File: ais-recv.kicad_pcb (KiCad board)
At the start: 4 copper layers, 40 x 20 mm, 44 parts, among them J1 Conn_02x05_Odd_Even, J2 CONSMA 003.062, J3 105017-0001, SW1 SW_Push, U1 NCP115ASN330T1G, U2 Si4362-C, U3 STM32L432KCUx, U4 USBLC6-2SC6, U5 Si4362-C, Y1 30 MHz

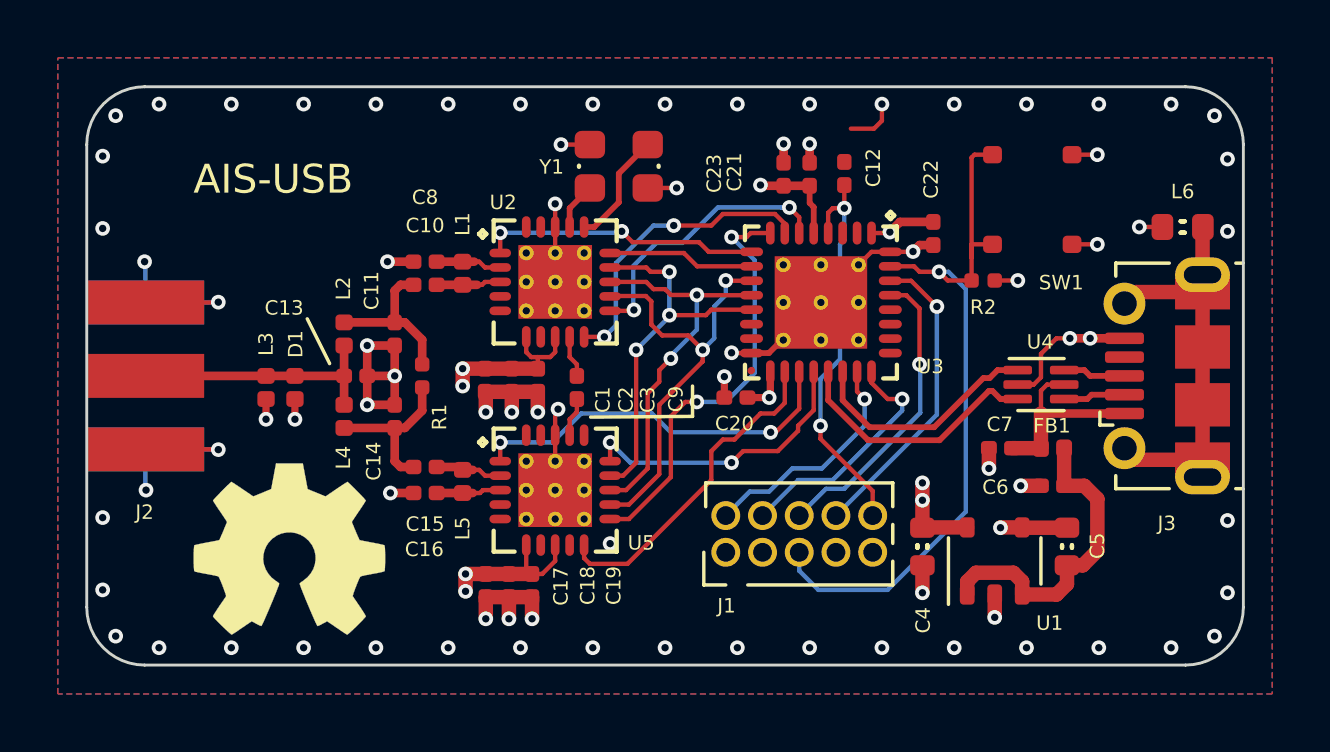
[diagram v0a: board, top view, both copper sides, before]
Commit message: Changes for version 1.0
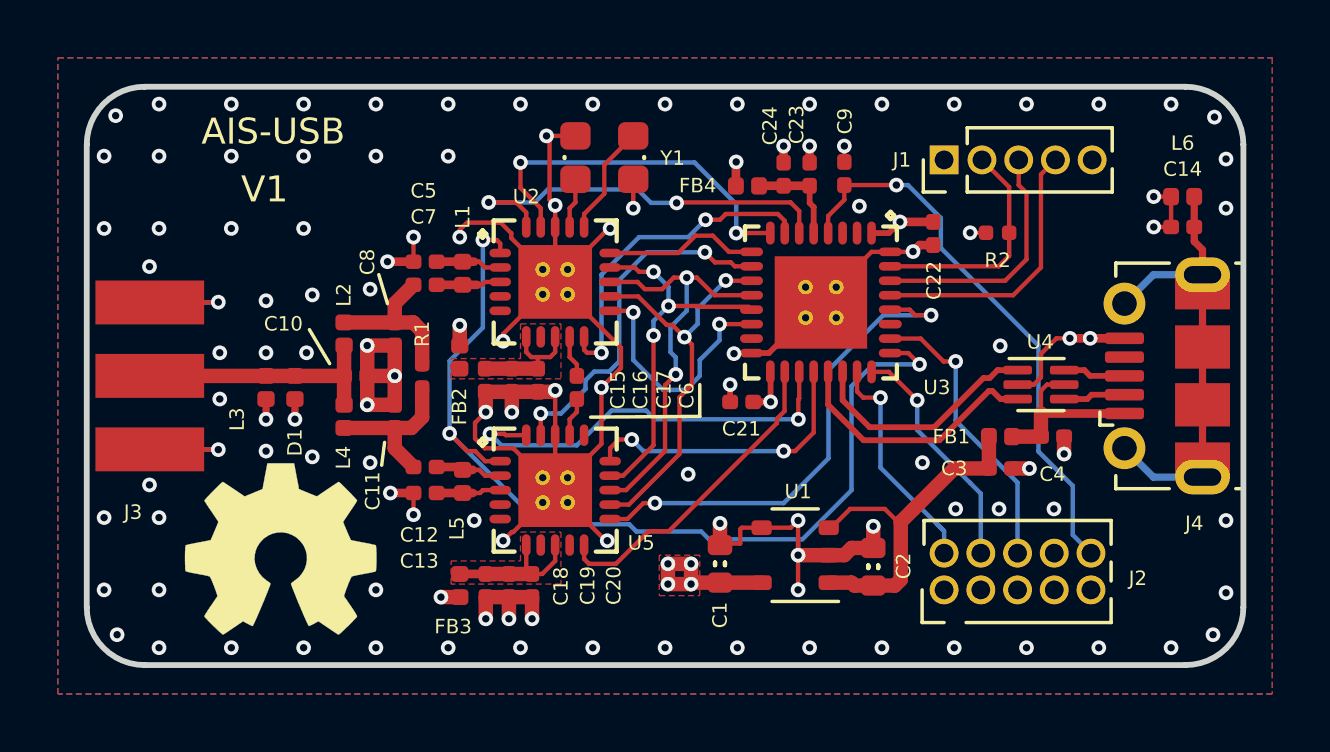
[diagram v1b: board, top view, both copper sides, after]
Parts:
- removed the C1 at (111.6, 91.2)
- removed SW1: SW_Push, local:SW_SPST_PTS_540
- added C14: DNP, IPC7351-Least:CAPC1005X55, F.Cu at (135.7, 85.8)
- added C15: 100pF, IPC7351-Least:CAPC1005X55, F.Cu at (111.6, 91.2)
- added FB2: 220 Ohm, IPC7351-Least:INDC1005X60, F.Cu at (110.7, 90.3)
- added FB3: 220 Ohm, IPC7351-Least:INDC1005X60, F.Cu at (110.7, 98.2)
- added FB4: 220 Ohm, IPC7351-Least:INDC1005X60, F.Cu at (120.7, 84.4)
- added J2: TMS-105-01-L-D, local:PinHeader_2x05_P1.27mm_Vertical, F.Cu at (127.5, 98.4)
- FB1: value Ferrite_Bead -> 220 Ohm
- J1: value Conn_02x05_Odd_Even -> FTS-105-01-L-S; footprint local:PinHeader_2x05_P1.27mm_Vertical -> Connector_PinHeader_1.27mm:PinHeader_1x05_P1.27mm_Vertical
- L3: value L -> 270 nH
- L6: footprint IPC7351-Least:INDC1608X95 -> IPC7351-Least:INDC1005X60
- moved J1 15.5 mm to (127.5, 83.5)
- moved C1 7.03 mm to (119.7, 97.5), turned to 90 degrees
- moved U1 6.90 mm to (122.3, 97.2), turned to 180 degrees
- moved C2 6.74 mm to (125.0, 97.6)
- moved C3 1.90 mm to (129.4, 94.2), turned to 0 degrees
- moved C4 1.84 mm to (131.2, 93.1), turned to 0 degrees
- moved FB1 1.84 mm to (129.4, 93.1), turned to 180 degrees
- moved R2 1.72 mm to (129.3, 86.0), turned to 180 degrees
- moved L6 1.05 mm to (135.7, 84.8)
- moved Y1 0.58 mm to (115.7, 83.5)
- moved LOGO1 0.30 mm to (104.5, 97.0)
- moved C21 0.25 mm to (120.5, 91.9)
- renumbered C4 to C1, C13 to C10, C14 to C11, C15 to C12, C16 to C13, C2 to C16, C3 to C17, C17 to C18, C18 to C19, C5 to C2, C19 to C20, C20 to C21, C21 to C23, C23 to C24, C6 to C3, C7 to C4, C8 to C5, C9 to C6, C10 to C7, C11 to C8, C12 to C9, J2 to J3, J3 to J4
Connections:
- C16 pad 1: VDD -> VDD_RF1
- C17 pad 1: VDD -> VDD_RF1
- C18 pad 1: VDD -> VDD_RF2
- C19 pad 1: VDD -> VDD_RF2
- C20 pad 1: VDD -> VDD_RF2
- C23 pad 1: VDD -> VDDA
- C24 pad 1: VDD -> VDDA
- J1 pad 2: SWDIO -> BOOT0
- J1 pad 3: GND -> UART1_RX
- J1 pad 4: SWDCLK -> UART1_TX
- J1 pad 5: /BOOT0 -> GND
- R2 pad 1: /BOOT0 -> BOOT0
- U2 pad 1: CH1_SDN -> SDN
- U2 pad 19: Net-(U2-Pad19) -> CH1_RX_CLK
- U2 pad 20: Net-(U2-Pad20) -> CH1_RX_DATA
- U2 pad 6: VDD -> VDD_RF1
- U2 pad 8: VDD -> VDD_RF1
- U3 pad 10: ~CH1_SEL -> CH2_RX_CLK
- U3 pad 14: Net-(U3-Pad14) -> ~CH1_IRQ
- U3 pad 19: CH2_SDN -> CH2_RX_DATA
- U3 pad 25: Net-(U3-Pad25) -> SDN
- U3 pad 26: Net-(U3-Pad26) -> SWO
- U3 pad 28: Net-(U3-Pad28) -> ~CH2_IRQ
- U3 pad 31: /BOOT0 -> BOOT0
- U3 pad 5: VDD -> VDDA
- U3 pad 6: ~CH1_IRQ -> CH1_RX_DATA
- U3 pad 8: ~CH2_IRQ -> CH1_RX_CLK
- U3 pad 9: CH1_SDN -> ~CH1_SEL
- U5 pad 1: CH2_SDN -> SDN
- U5 pad 19: Net-(U5-Pad19) -> CH2_RX_CLK
- U5 pad 20: Net-(U5-Pad20) -> CH2_RX_DATA
- U5 pad 6: VDD -> VDD_RF2
- U5 pad 8: VDD -> VDD_RF2
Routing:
- net GND: track 62.8 -> 100.7 mm, vias 78 -> 121
- net SDN: track 0.00 -> 33.8 mm, vias 0 -> 3
- net /BOOT0: track 25.8 -> 0.00 mm, vias 1 -> 0
- net CH2_RX_DATA: track 0.00 -> 14.4 mm, vias 0 -> 2
- net CH1_RX_DATA: track 0.00 -> 14.0 mm, vias 0 -> 2
- net CH2_SDN: track 13.3 -> 0.00 mm, vias 2 -> 0
- net CH1_RX_CLK: track 0.00 -> 12.8 mm, vias 0 -> 2
- net CH2_RX_CLK: track 0.00 -> 12.4 mm, vias 0 -> 2
- net VDD: track 23.7 -> 11.8 mm, vias 11 -> 9
- net SWO: track 0.00 -> 10.1 mm, vias 0 -> 1
- net CH1_SDN: track 9.70 -> 0.00 mm, vias 2 -> 0
- net BOOT0: track 0.00 -> 7.97 mm
- net ~RESET: track 13.8 -> 19.4 mm, vias 2 -> 1
- net VDD_RF2: track 0.00 -> 5.12 mm
- net VDD_RF1: track 0.00 -> 4.41 mm
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- added copper zone on F.Cu, net VDD
- added copper zone on F.Cu, net VDD_RF1
- added copper zone on F.Cu, net VDD_RF2
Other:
- rule pad_to_mask_clearance: 0.051 -> 0.0381
- board text added: "BOOT0"
- board text added: "GND"
- board text added: "RX"
- board text added: "TX"
- board text added: "V1"
- board text added: "VDD"
